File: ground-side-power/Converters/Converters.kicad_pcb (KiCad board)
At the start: 2 copper layers, 32 parts, among them J10 Conn_01x03_Female, J11 Conn_01x03_Female, J12 Conn_01x04_Female, J13 DAQ Voltage Sensing, J14 DAQ Current Sensing, J27 Conn_01x02_Female, U3 K7805-3AR3, U4 INA180, U5 INA180, U6 URB2424LD-20WR3

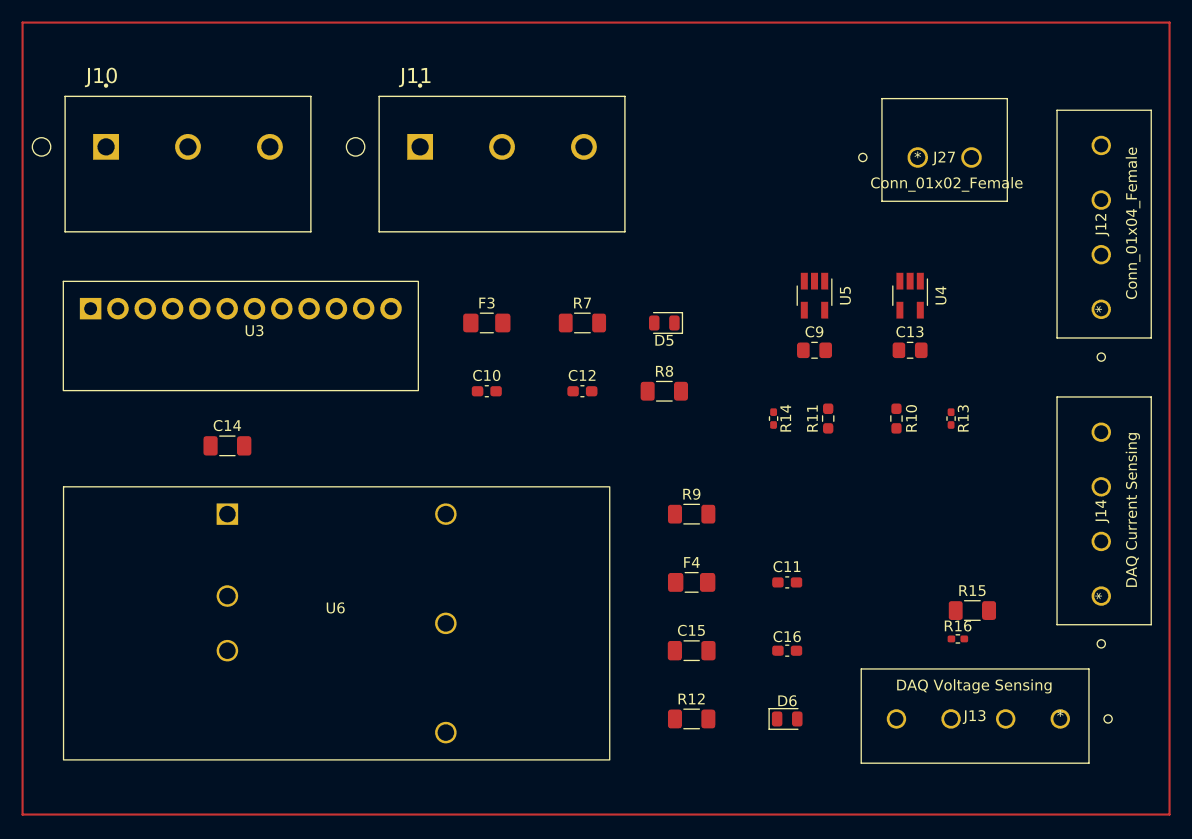
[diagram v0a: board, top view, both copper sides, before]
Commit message: PCB Layout First Draft
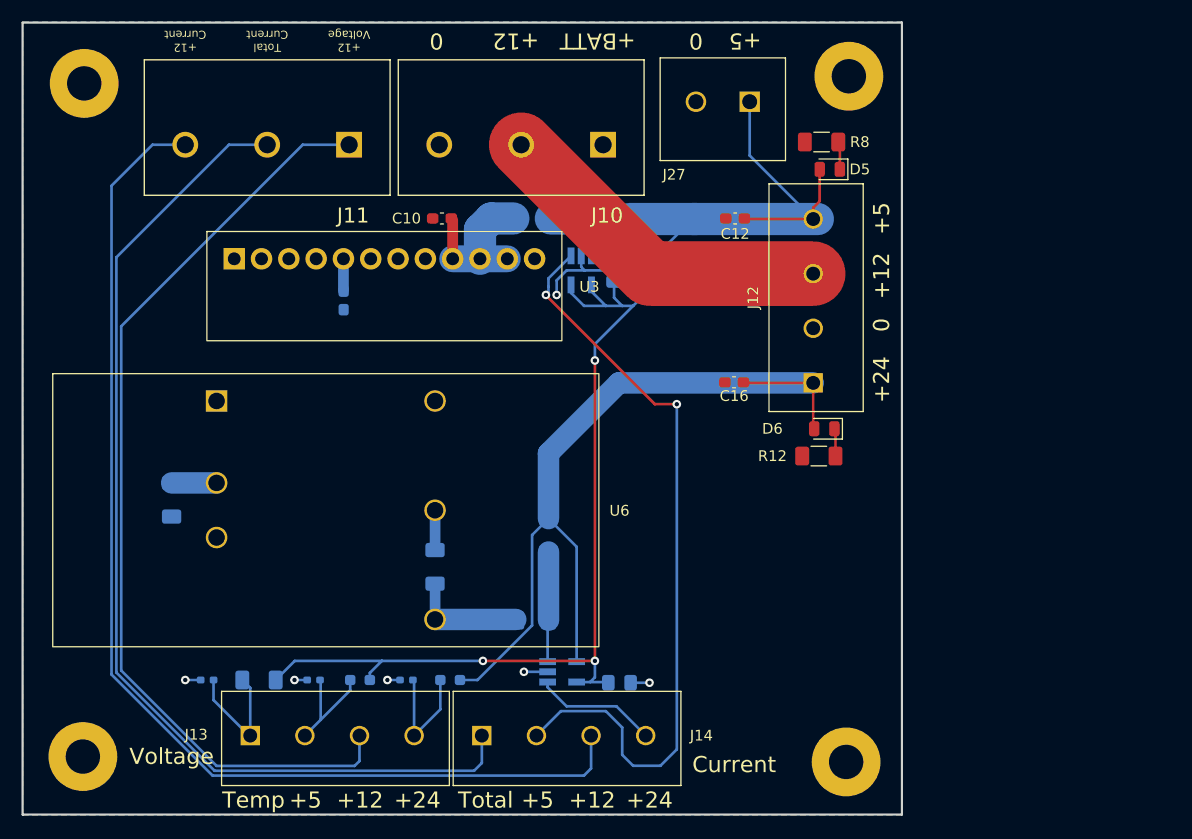
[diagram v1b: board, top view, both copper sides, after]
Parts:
- added ?: , clipboard:6b5716c7-8553-4764-af17-05841c85de2e, F.Cu at (152.4, 68.7)
- added ?: , clipboard:6b5716c7-8553-4764-af17-05841c85de2e, F.Cu at (152.1, 132.5)
- added ?: , clipboard:6b5716c7-8553-4764-af17-05841c85de2e, F.Cu at (81.2, 132.0)
- added ?: , clipboard:6b5716c7-8553-4764-af17-05841c85de2e, F.Cu at (81.3, 69.3)
- C11, C13, C14, C15, C9, F3, F4, R10, R11, R13, R14, R15, R16, R7, R9, U4, U5: moved to B.Cu
- moved J13 75.4 mm to (96.7, 134.2), turned to 0 degrees
- moved R16 69.9 mm to (92.7, 129.0), turned to 180 degrees
- moved R15 66.7 mm to (97.5, 129.0), turned to 180 degrees
- moved J14 59.1 mm to (118.3, 134.2), turned to 0 degrees
- moved R13 56.2 mm to (111.3, 129.0), turned to 180 degrees
- moved R11 49.9 mm to (106.9, 129.0), turned to 180 degrees
- moved R14 49.2 mm to (102.6, 129.0), turned to 180 degrees
- moved C11 48.9 mm to (105.4, 93.7), turned to 90 degrees
- moved R10 48.1 mm to (115.3, 129.0), turned to 180 degrees
- moved J10 46.2 mm to (129.5, 79.2), turned to 180 degrees
- moved U5 42.1 mm to (125.7, 128.3), turned to 0 degrees
- moved C13 41.1 mm to (131.1, 129.3), turned to 180 degrees
- moved U4 30.7 mm to (127.5, 90.9)
- moved J12 27.7 mm to (149.1, 101.4)
- moved R8 27.4 mm to (149.9, 79.0)
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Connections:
- J11 pad 1: /12V_OUT -> /12_VOLTAGE
- J11 pad 3: /12_VOLTAGE -> /12V_OUT
- J12 pad 1: +5V -> +24V
- J12 pad 2: /+12V -> GND
- J12 pad 3: +24V -> /+12V
- J12 pad 4: GND -> +5V
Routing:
- net +5V: track 0.00 -> 137.9 mm, vias 0 -> 3
- net /12V_OUT: track 0.00 -> 105.7 mm
- net /TOTAL_OUT: track 0.00 -> 96.9 mm
- net /12_VOLTAGE: track 0.00 -> 87.9 mm
- net +24V: track 0.00 -> 78.0 mm
- net /5V_OUT: track 0.00 -> 71.3 mm, vias 0 -> 2
- net /+12V: track 0.00 -> 32.1 mm
- net GND: track 0.00 -> 27.7 mm, vias 0 -> 6
- net Net-(C10-Pad1): track 0.00 -> 15.8 mm
- net /Temp: track 0.00 -> 12.1 mm
- net /24V_OUT: track 0.00 -> 11.5 mm
- net /24V_VOLTAGE: track 0.00 -> 11.4 mm
- net Net-(C15-Pad1): track 0.00 -> 10.9 mm
- net /5V_VOLTAGE: track 0.00 -> 10.6 mm
- net /24V_Sense+: track 0.00 -> 10.2 mm
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- added copper zone on B.Cu, net +BATT
- added copper zone on F.Cu, net GND
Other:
- board outline added: 81.8 x 73.7 mm
- board text added: "+12"
- board text added: "+12 Current"
- board text added: "+12 Voltage"
- board text added: "+24"
- board text added: "+5"
- board text added: "+BATT"
- board text added: "0"
- board text added: "Current"
- board text added: "Temp"
- board text added: "Total"
- board text added: "Total Current"
- board text added: "Voltage"
